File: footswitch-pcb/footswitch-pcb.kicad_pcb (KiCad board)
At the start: 2 copper layers, 14 parts, among them J1 Conn_Pedal, J2 Solder_Pad_BAT+, J3 Solder_Pad_Reset, J4 Conn_01x02_Male, J5 Solder_Pad_BAT-, SW1 SW_DIP_x03, SW2 SW_BLUETOOTH, SW3 SW_RESET, U1 SeeeduinoXIAO

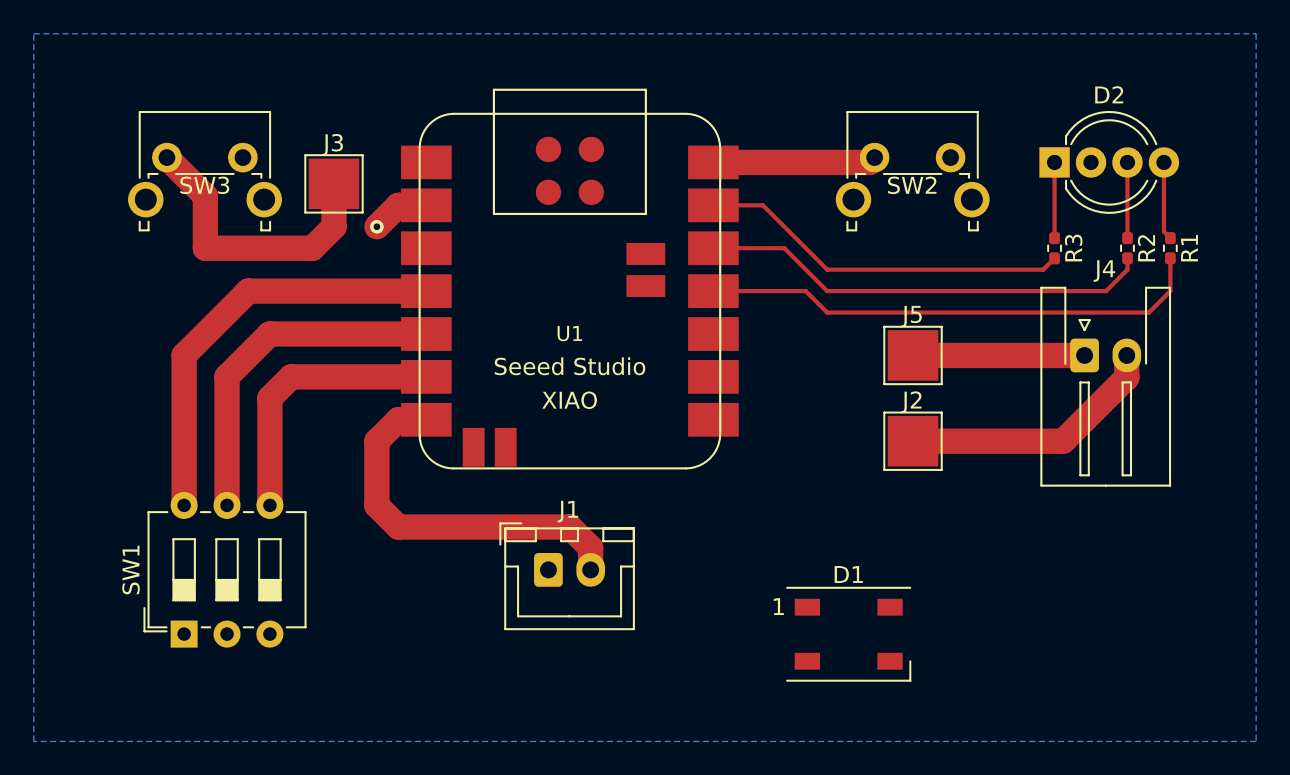
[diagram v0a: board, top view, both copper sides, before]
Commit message: PCB update
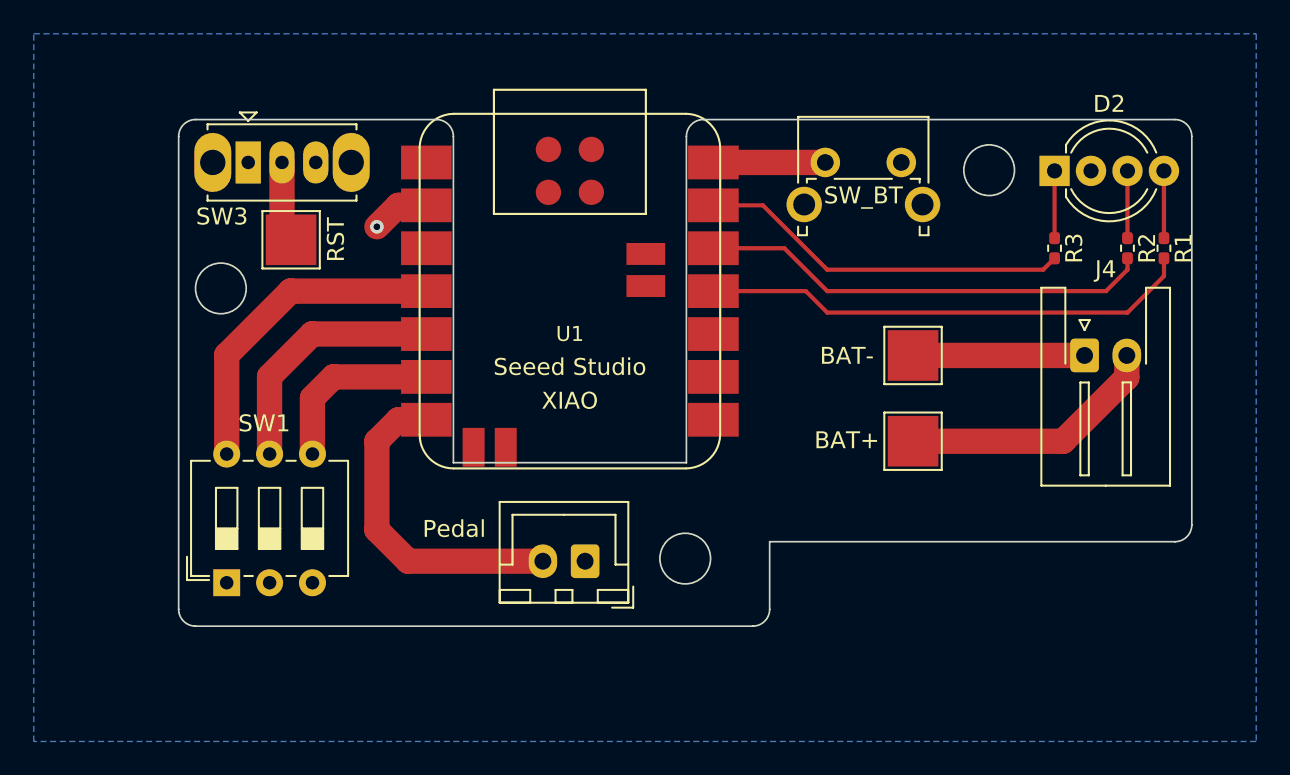
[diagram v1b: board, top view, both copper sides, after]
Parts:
- removed D1: WS2812B, LED_SMD:LED_WS2812B_PLCC4_5.0x5.0mm_P3.2mm
- SW3: value SW_RESET -> SW_SPDT; footprint Button_Switch_THT:SW_Tactile_SPST_Angled_PTS645Vx39-2LFS -> Button_Switch_THT:SW_Slide_1P2T_CK_OS102011MS2Q
- moved SW3 4.82 mm to (114.3, 73.7)
- moved RST 4.17 mm to (116.8, 78.2), turned to 90 degrees
- moved SW1 3.95 mm to (113.0, 98.5)
- moved SW_BT 2.93 mm to (148.5, 73.7)
- moved Pedal 2.23 mm to (134.2, 97.3), turned to 180 degrees
- moved D2 0.50 mm to (162.1, 74.2)
- moved R1 0.38 mm to (168.5, 78.7)
- renumbered J2 to BAT+, J5 to BAT-, J1 to Pedal, J3 to RST, SW2 to SW_BT
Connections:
- SW3 pad 1: Net-(J3-Pad1) -> unconnected-(SW3-Pad1)
- SW3 pad 2: GND -> Net-(J3-Pad1)
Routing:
- net Net-(J3-Pad1): track 17.0 -> 4.80 mm
- net PIN_LAYER2: track 20.5 -> 15.0 mm
- net PIN_LAYER3: track 16.2 -> 10.6 mm
- net PIN_LAYER1: track 24.8 -> 19.3 mm
- net PIN_BT: track 9.66 -> 6.62 mm
- net PIN_PEDAL: track 22.3 -> 19.3 mm
- net PIN_LEDB: track 30.1 -> 29.2 mm
- net Net-(D2-Pad4): track 4.64 -> 3.98 mm
- net Net-(D2-Pad3): track 4.48 -> 3.98 mm
- net Net-(D2-Pad1): track 4.48 -> 3.98 mm
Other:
- board outline added: 60 x 30 mm
